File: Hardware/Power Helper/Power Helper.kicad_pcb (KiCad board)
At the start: 2 copper layers, 54.3 x 27 mm, 15 parts, among them J1 USB_C_Receptacle_Power_Only, J2 Conn_02x02_Odd_Even, J3 Conn_02x02_Odd_Even, SW1 SW_SPDT, SW2 SW_SPDT, SW3 SW_SPDT, U1 AZ1117-3.3

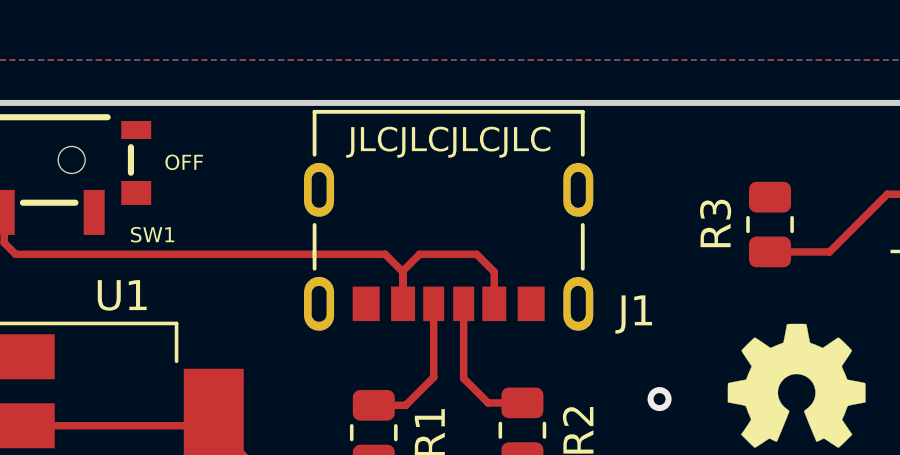
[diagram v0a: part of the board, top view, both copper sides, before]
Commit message: Add LED helper
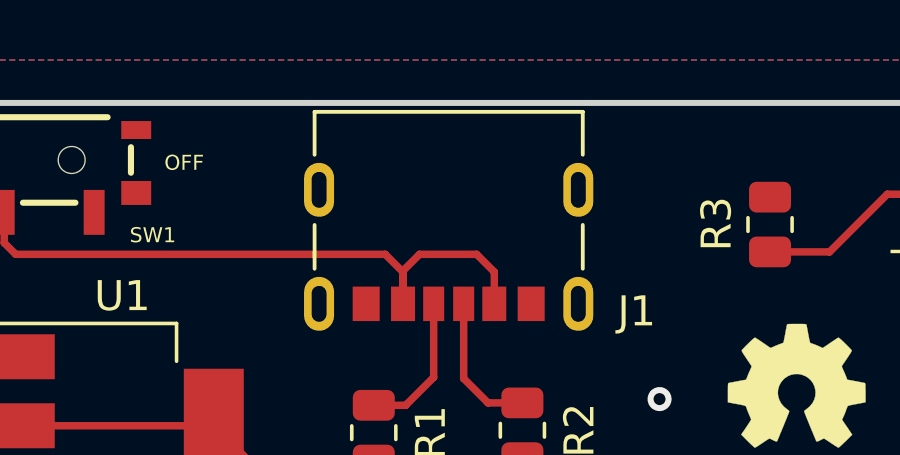
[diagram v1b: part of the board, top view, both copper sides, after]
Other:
- board text removed: "JLCJLCJLCJLC"
